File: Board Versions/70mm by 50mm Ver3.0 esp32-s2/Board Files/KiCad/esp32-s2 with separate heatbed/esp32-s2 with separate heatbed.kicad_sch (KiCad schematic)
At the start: 59 parts, among them IC1 ESP32-S2FN4R2, J1 PJ-037B, J2 USB4520-03-0-A, J3 TB003-500-P02BE, J4 TB003-500-P02BE, Q1 PJD25N06A_L2_00001, U1 LD1117S33TR_SOT223, U2 MAX31855KASA, Y1 ECS-400-15-33B-CTN-TR

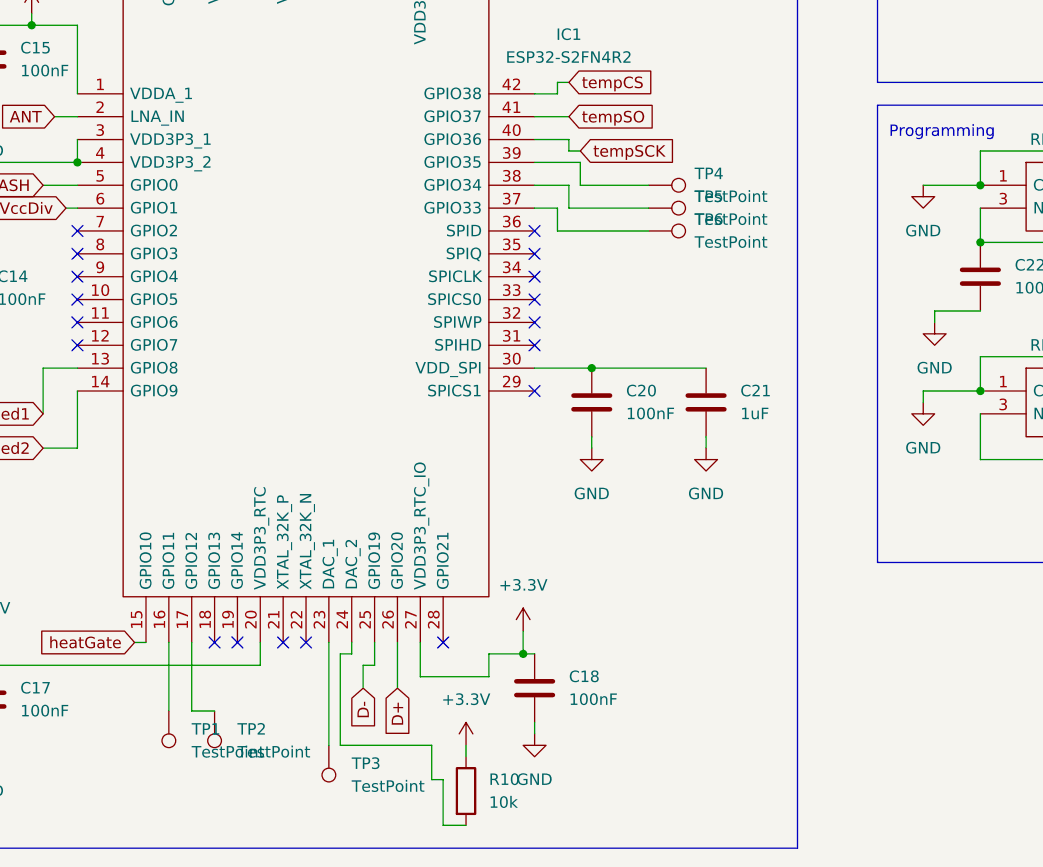
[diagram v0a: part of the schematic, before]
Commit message: Routing complete
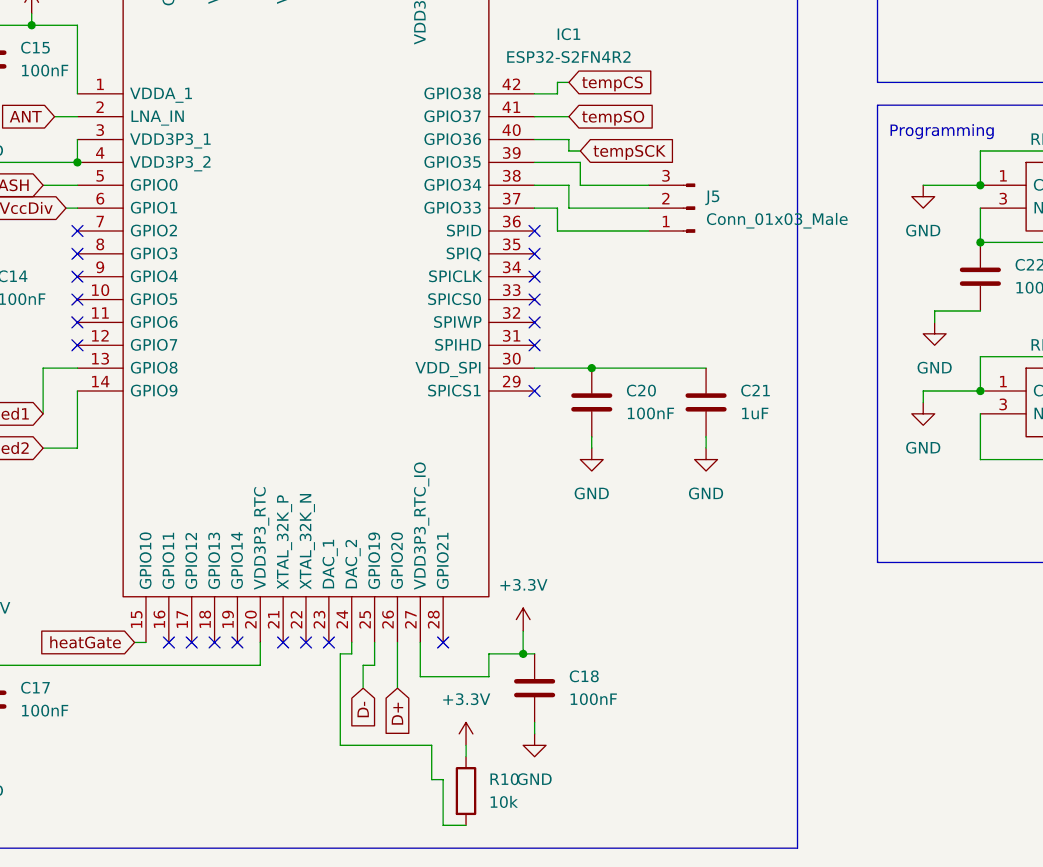
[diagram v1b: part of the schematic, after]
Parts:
- removed TP1, TP2, TP3, TP4, TP5, TP6: TestPoint, Connector_PinHeader_2.54mm:PinHeader_1x01_P2.54mm_Vertical, symbol Connector:TestPoint
- added J5: Conn_01x03_Male, Connector_PinHeader_2.54mm:PinHeader_1x03_P2.54mm_Vertical, symbol Connector:Conn_01x03_Male
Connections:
- net at IC1.39 (GPIO35): now also J5.3 (Pin_3)
- net at IC1.37 (GPIO33): now also J5.1 (Pin_1)
- net at IC1.38 (GPIO34): now also J5.2 (Pin_2)
- no-connect marks 32 -> 35
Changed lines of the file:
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@@
   (no_connect (at 95.25 134.62))
   (no_connect (at 95.25 137.16))
-  (no_connect (at 113.03 170.18))
   (no_connect (at 110.49 170.18))
+  (no_connect (at 113.03 170.18))
+  (no_connect (at 123.19 170.18))
+  (no_connect (at 107.95 170.18))
+  (no_connect (at 105.41 170.18))
   (no_connect (at 146.05 124.46))
   (no_connect (at 146.05 127))
@@
     (stroke (width 0) (type default) (color 0 0 0 0))
   )
-  (wire (pts (xy 123.19 170.18) (xy 123.19 181.61))
-    (stroke (width 0) (type default) (color 0 0 0 0))
-  )
   (wire (pts (xy 21.59 90.17) (xy 21.59 102.87))
     (stroke (width 0) (type default) (color 0 0 0 0))
@@
     (stroke (width 0) (type default) (color 0 0 0 0))
   )
-  (wire (pts (xy 105.41 170.18) (xy 105.41 177.8))
-    (stroke (width 0) (type default) (color 0 0 0 0))
-  )
   (wire (pts (xy 25.4 161.29) (xy 35.56 161.29))
     (stroke (width 0) (type default) (color 0 0 0 0))
@@
     (stroke (width 0) (type default) (color 0 0 0 0))
   )
-  (wire (pts (xy 107.95 177.8) (xy 107.95 170.18))
-    (stroke (width 0) (type default) (color 0 0 0 0))
-  )
   (wire (pts (xy 67.31 21.59) (xy 67.31 27.94))
     (stroke (width 0) (type default) (color 0 0 0 0))
@@
     (stroke (width 0) (type default) (color 0 0 0 0))
   )
-  (wire (pts (xy 110.49 177.8) (xy 107.95 177.8))
-    (stroke (width 0) (type default) (color 0 0 0 0))
-  )
   (wire (pts (xy 132.08 40.64) (xy 135.89 40.64))
     (stroke (width 0) (type default) (color 0 0 0 0))
@@
     (pin "1")
   )
-  (symbol (lib_id "Connector:TestPoint") (at 105.41 177.8 180) (unit 1)
-    (in_bom yes) (on_board yes) (fields_autoplaced)
-    (property "Reference" "TP1" (id 0) (at 107.95 179.8319 0)
-      (effects (font (size 1.27 1.27)) (justify right))
-    )
-    (property "Value" "TestPoint" (id 1) (at 107.95 182.3719 0)
-      (effects (font (size 1.27 1.27)) (justify right))
-    )
-    (property "Footprint" "Connector_PinHeader_2.54mm:PinHeader_1x01_P2.54mm_Vertical" (id 2) (at 100.33 177.8 0)
-      (effects (font (size 1.27 1.27)) hide)
-    )
-    (property "Datasheet" "~" (id 3) (at 100.33 177.8 0)
-      (effects (font (size 1.27 1.27)) hide)
-    )
-    (pin "1")
-  )
   (symbol (lib_id "Device:R") (at 260.35 144.78 0) (unit 1)
     (in_bom yes) (on_board yes) (fields_autoplaced)
@@
     (pin "2")
   )
-  (symbol (lib_id "Connector:TestPoint") (at 158.75 119.38 270) (unit 1)
-    (in_bom yes) (on_board yes) (fields_autoplaced)
-    (property "Reference" "TP4" (id 0) (at 163.83 118.1099 90)
-      (effects (font (size 1.27 1.27)) (justify left))
-    )
-    (property "Value" "TestPoint" (id 1) (at 163.83 120.6499 90)
-      (effects (font (size 1.27 1.27)) (justify left))
-    )
-    (property "Footprint" "Connector_PinHeader_2.54mm:PinHeader_1x01_P2.54mm_Vertical" (id 2) (at 158.75 124.46 0)
-      (effects (font (size 1.27 1.27)) hide)
-    )
-    (property "Datasheet" "~" (id 3) (at 158.75 124.46 0)
-      (effects (font (size 1.27 1.27)) hide)
-    )
-    (pin "1")
-  )
   (symbol (lib_id "power:+3.3V") (at 167.64 36.83 0) (unit 1)
     (in_bom yes) (on_board yes) (fields_autoplaced)
@@
     (pin "2")
   )
-  (symbol (lib_id "Connector:TestPoint") (at 110.49 177.8 180) (unit 1)
-    (in_bom yes) (on_board yes) (fields_autoplaced)
-    (property "Reference" "TP2" (id 0) (at 113.03 179.8319 0)
-      (effects (font (size 1.27 1.27)) (justify right))
-    )
-    (property "Value" "TestPoint" (id 1) (at 113.03 182.3719 0)
-      (effects (font (size 1.27 1.27)) (justify right))
-    )
-    (property "Footprint" "Connector_PinHeader_2.54mm:PinHeader_1x01_P2.54mm_Vertical" (id 2) (at 105.41 177.8 0)
-      (effects (font (size 1.27 1.27)) hide)
-    )
-    (property "Datasheet" "~" (id 3) (at 105.41 177.8 0)
-      (effects (font (size 1.27 1.27)) hide)
-    )
-    (pin "1")
-  )
   (symbol (lib_id "Device:C") (at 83.82 38.1 0) (unit 1)
     (in_bom yes) (on_board yes) (fields_autoplaced)
@@
     (pin "1")
   )
-  (symbol (lib_id "Connector:TestPoint") (at 158.75 124.46 270) (unit 1)
-    (in_bom yes) (on_board yes) (fields_autoplaced)
-    (property "Reference" "TP6" (id 0) (at 163.83 123.1899 90)
-      (effects (font (size 1.27 1.27)) (justify left))
-    )
-    (property "Value" "TestPoint" (id 1) (at 163.83 125.7299 90)
-      (effects (font (size 1.27 1.27)) (justify left))
-    )
-    (property "Footprint" "Connector_PinHeader_2.54mm:PinHeader_1x01_P2.54mm_Vertical" (id 2) (at 158.75 129.54 0)
-      (effects (font (size 1.27 1.27)) hide)
-    )
-    (property "Datasheet" "~" (id 3) (at 158.75 129.54 0)
-      (effects (font (size 1.27 1.27)) hide)
-    )
-    (pin "1")
-  )
   (symbol (lib_id "library_loader:PJ-037B") (at 33.02 40.64 180) (unit 1)
     (in_bom yes) (on_board yes) (fields_autoplaced)
@@
     (pin "1")
   )
-  (symbol (lib_id "Connector:TestPoint") (at 158.75 121.92 270) (unit 1)
-    (in_bom yes) (on_board yes) (fields_autoplaced)
-    (property "Reference" "TP5" (id 0) (at 163.83 120.6499 90)
-      (effects (font (size 1.27 1.27)) (justify left))
-    )
-    (property "Value" "TestPoint" (id 1) (at 163.83 123.1899 90)
-      (effects (font (size 1.27 1.27)) (justify left))
-    )
-    (property "Footprint" "Connector_PinHeader_2.54mm:PinHeader_1x01_P2.54mm_Vertical" (id 2) (at 158.75 127 0)
-      (effects (font (size 1.27 1.27)) hide)
-    )
-    (property "Datasheet" "~" (id 3) (at 158.75 127 0)
-      (effects (font (size 1.27 1.27)) hide)
-    )
-    (pin "1")
-  )
   (symbol (lib_id "Device:R") (at 27.94 80.01 0) (unit 1)
     (in_bom yes) (on_board yes) (fields_autoplaced)
@@
     (pin "1")
   )
+  (symbol (lib_id "Connector:Conn_01x03_Male") (at 163.83 121.92 180) (unit 1)
+    (in_bom yes) (on_board yes) (fields_autoplaced)
+    (property "Reference" "J5" (id 0) (at 165.1 120.6499 0)
+      (effects (font (size 1.27 1.27)) (justify right))
+    )
+    (property "Value" "Conn_01x03_Male" (id 1) (at 165.1 123.1899 0)
+      (effects (font (size 1.27 1.27)) (justify right))
+    )
+    (property "Footprint" "Connector_PinHeader_2.54mm:PinHeader_1x03_P2.54mm_Vertical" (id 2) (at 163.83 121.92 0)
+      (effects (font (size 1.27 1.27)) hide)
+    )
+    (property "Datasheet" "~" (id 3) (at 163.83 121.92 0)
+      (effects (font (size 1.27 1.27)) hide)
+    )
+    (pin "1")
+    (pin "2")
+    (pin "3")
+  )
   (symbol (lib_id "power:GND") (at 92.71 83.82 0) (unit 1)
     (in_bom yes) (on_board yes) (fields_autoplaced)
@@
     (pin "1")
   )
-  (symbol (lib_id "Connector:TestPoint") (at 123.19 181.61 180) (unit 1)
-    (in_bom yes) (on_board yes) (fields_autoplaced)
-    (property "Reference" "TP3" (id 0) (at 125.73 183.6419 0)
-      (effects (font (size 1.27 1.27)) (justify right))
-    )
-    (property "Value" "TestPoint" (id 1) (at 125.73 186.1819 0)
-      (effects (font (size 1.27 1.27)) (justify right))
-    )
-    (property "Footprint" "Connector_PinHeader_2.54mm:PinHeader_1x01_P2.54mm_Vertical" (id 2) (at 118.11 181.61 0)
-      (effects (font (size 1.27 1.27)) hide)
-    )
-    (property "Datasheet" "~" (id 3) (at 118.11 181.61 0)
-      (effects (font (size 1.27 1.27)) hide)
-    )
-    (pin "1")
-  )
   (symbol (lib_id "power:GND") (at 24.13 78.74 0) (unit 1)
     (in_bom yes) (on_board yes) (fields_autoplaced)
@@
       (reference "J4") (unit 1) (value "TB003-500-P02BE") (footprint "library_manager:SHDR2W100P0X500_1X2_1000X780X1030P")
     )
+    (path "/ad6cfbb5-6560-4e8d-b51f-2fc576abbdaf"
+      (reference "J5") (unit 1) (value "Conn_01x03_Male") (footprint "Connector_PinHeader_2.54mm:PinHeader_1x03_P2.54mm_Vertical")
+    )
     (path "/4cebe0d3-dd69-4a3c-8afb-1f7ed5f46b3f"
       (reference "Q1") (unit 1) (value "PJD25N06A_L2_00001") (footprint "library_manager:PJD25N06A_L2_00001")
@@
       (reference "S2") (unit 1) (value "RKC2SJF170SMTR_LFS") (footprint "library_manager:RKC2SJF170SMTRLFS")
     )
-    (path "/11193139-e627-47b8-acb2-c7465a48e18b"
-      (reference "TP1") (unit 1) (value "TestPoint") (footprint "Connector_PinHeader_2.54mm:PinHeader_1x01_P2.54mm_Vertical")
-    )
-    (path "/4967b1ed-cf9b-4db7-9bd1-e8a2d70f4a53"
-      (reference "TP2") (unit 1) (value "TestPoint") (footprint "Connector_PinHeader_2.54mm:PinHeader_1x01_P2.54mm_Vertical")
-    )
-    (path "/e1996bfa-6f33-4144-b3b8-0ecaa63a9bf1"
-      (reference "TP3") (unit 1) (value "TestPoint") (footprint "Connector_PinHeader_2.54mm:PinHeader_1x01_P2.54mm_Vertical")
-    )
-    (path "/3806a371-9c6c-48e3-8acc-c75ec9bc196b"
-      (reference "TP4") (unit 1) (value "TestPoint") (footprint "Connector_PinHeader_2.54mm:PinHeader_1x01_P2.54mm_Vertical")
-    )
-    (path "/929d007f-ac7c-4a9f-b46d-d6c7bd0e649e"
-      (reference "TP5") (unit 1) (value "TestPoint") (footprint "Connector_PinHeader_2.54mm:PinHeader_1x01_P2.54mm_Vertical")
-    )
-    (path "/8c3d3de0-d23f-45b0-b638-d3824cb5c779"
-      (reference "TP6") (unit 1) (value "TestPoint") (footprint "Connector_PinHeader_2.54mm:PinHeader_1x01_P2.54mm_Vertical")
-    )
     (path "/db94c8fc-a32f-4093-9a65-a86b21b63695"
